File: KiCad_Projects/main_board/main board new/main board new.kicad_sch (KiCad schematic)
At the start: 76 parts

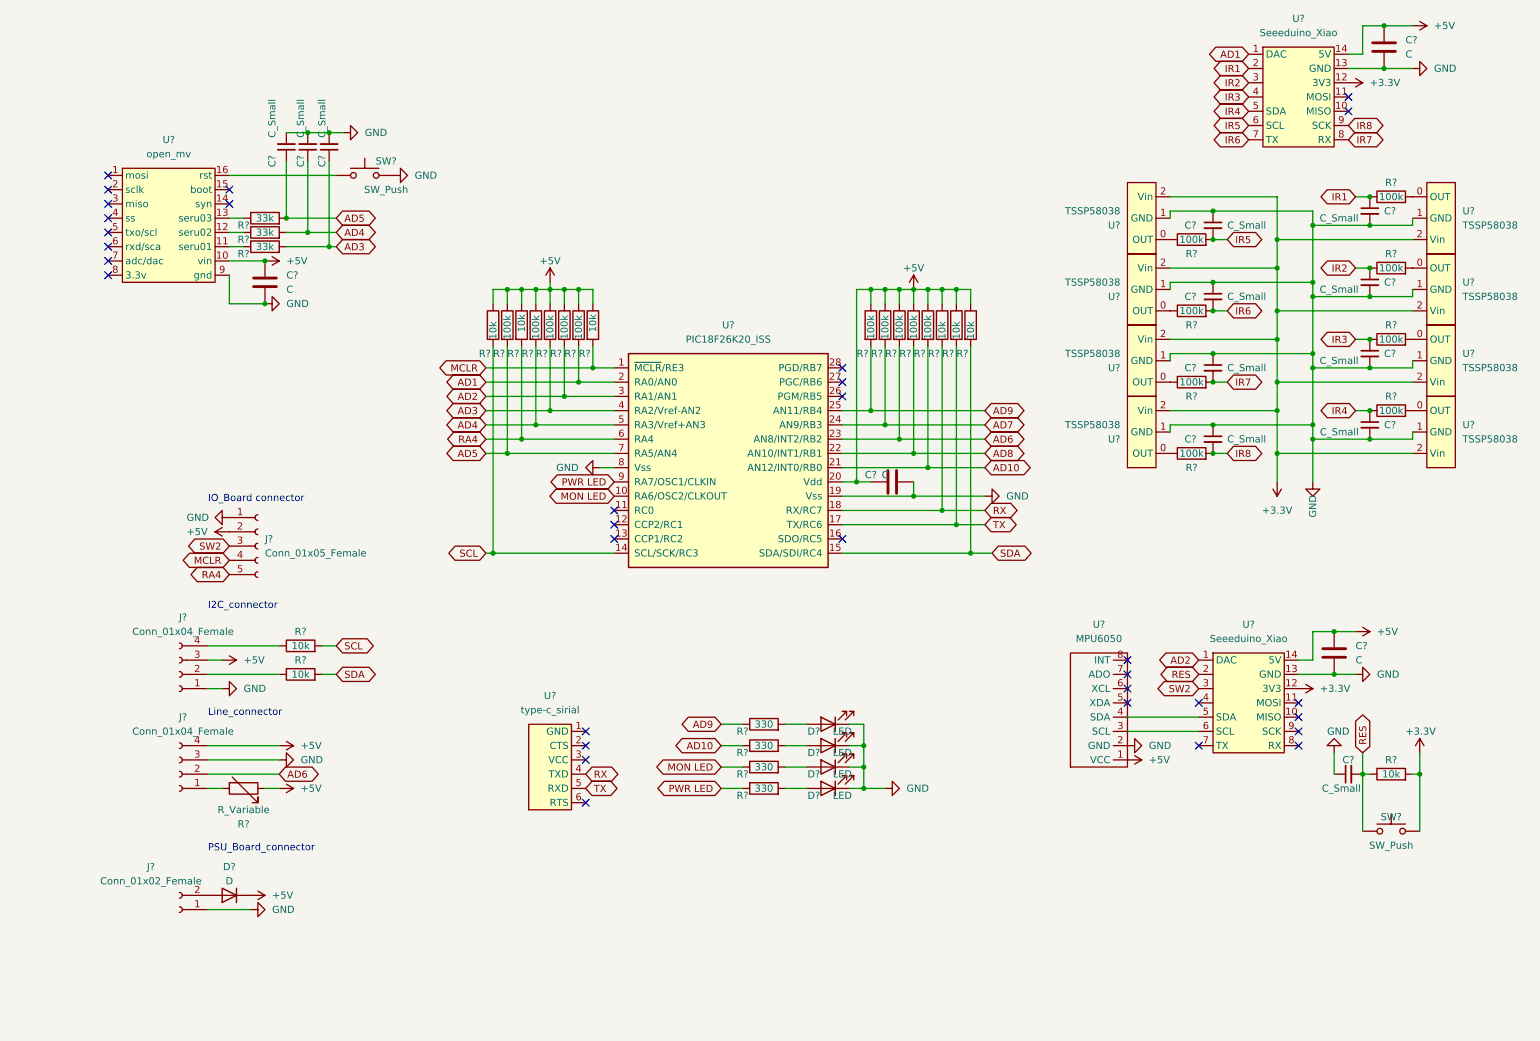
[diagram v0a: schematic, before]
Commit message: 基板データの更新
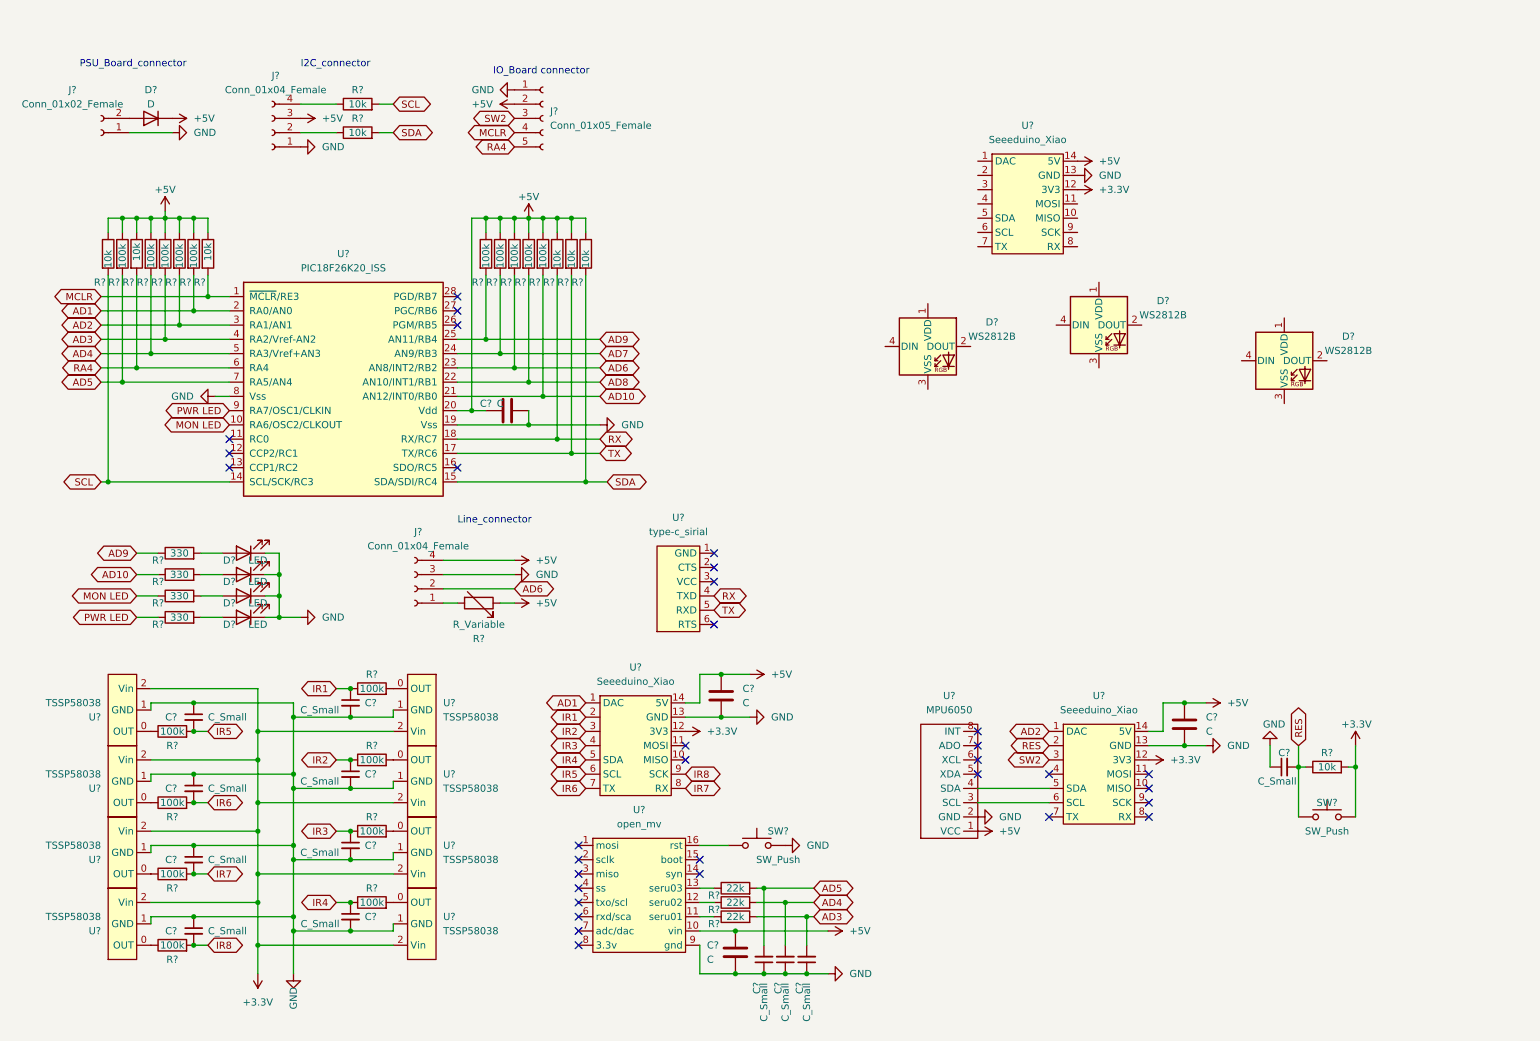
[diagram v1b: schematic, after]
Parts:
- removed C? (x3): C_Small, Capacitor_THT:C_Disc_D3.8mm_W2.6mm_P2.50mm, symbol Device:C_Small
- added C? (x3): C_Small, Capacitor_THT:C_Disc_D3.8mm_W2.6mm_P2.50mm, symbol Device:C_Small
- added D? (x3): WS2812B, LED_SMD:LED_WS2812B_PLCC4_5.0x5.0mm_P3.2mm, symbol LED:WS2812B
- added U?: Seeeduino_Xiao, Lib:seeeduinoXIAO, symbol seeeduino_xiao:Seeeduino_Xiao
- R? (x3): value 33k -> 22k
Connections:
- net +3V3: now also U?.12 (3V3)
- net +5V: now also U?.14 (5V)
- net AD3: now also C?.2
- net AD4: now also C?.2
- net AD5: now also C?.2
- net GND: now also C?.1, C?.1, C?.1, U?.13 (GND)
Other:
- moved on the sheet: C?, D?, J?, R?, SW?, U?
